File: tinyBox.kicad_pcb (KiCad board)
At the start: 2 copper layers, 29 x 20 mm, 15 parts, among them J1 USB_B_Micro, SW1 SW_DIP_x01, U1 ATSAMD21E15A-M, U2 AP2112K-3.3

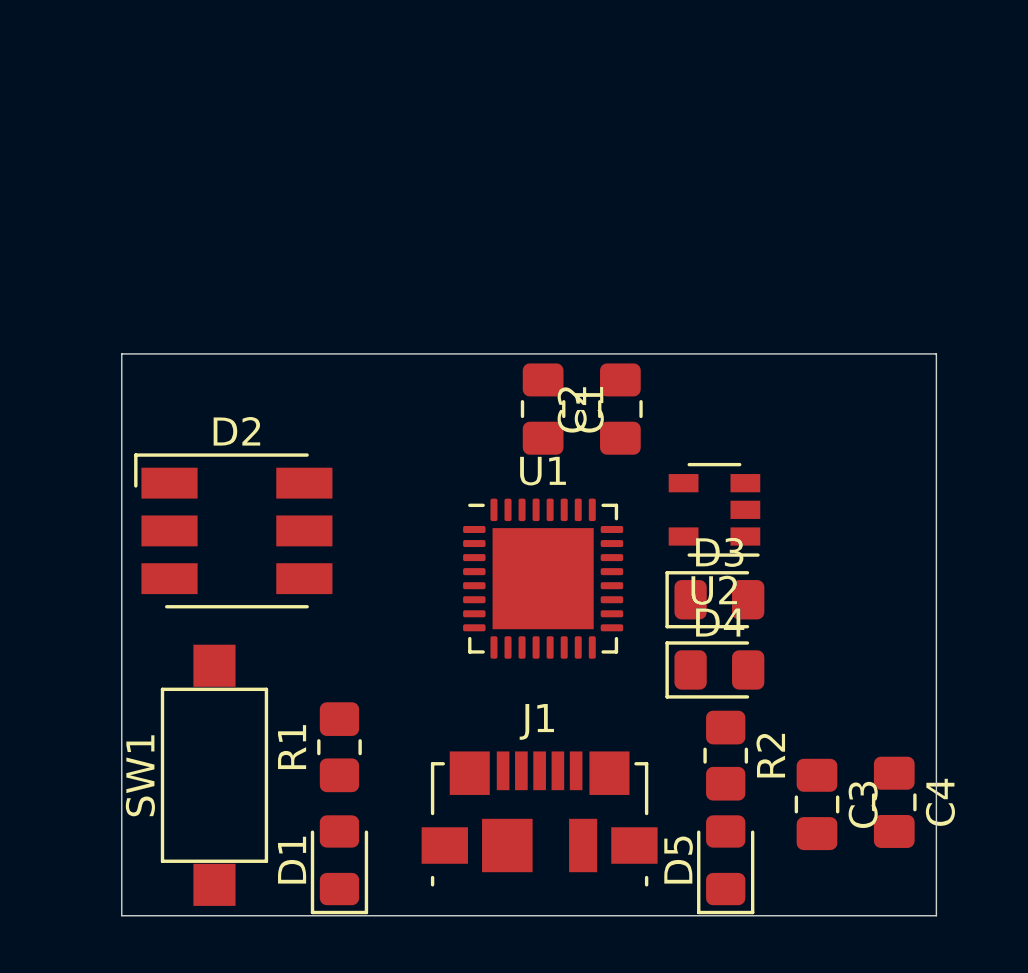
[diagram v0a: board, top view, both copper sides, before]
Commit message: Add files via upload
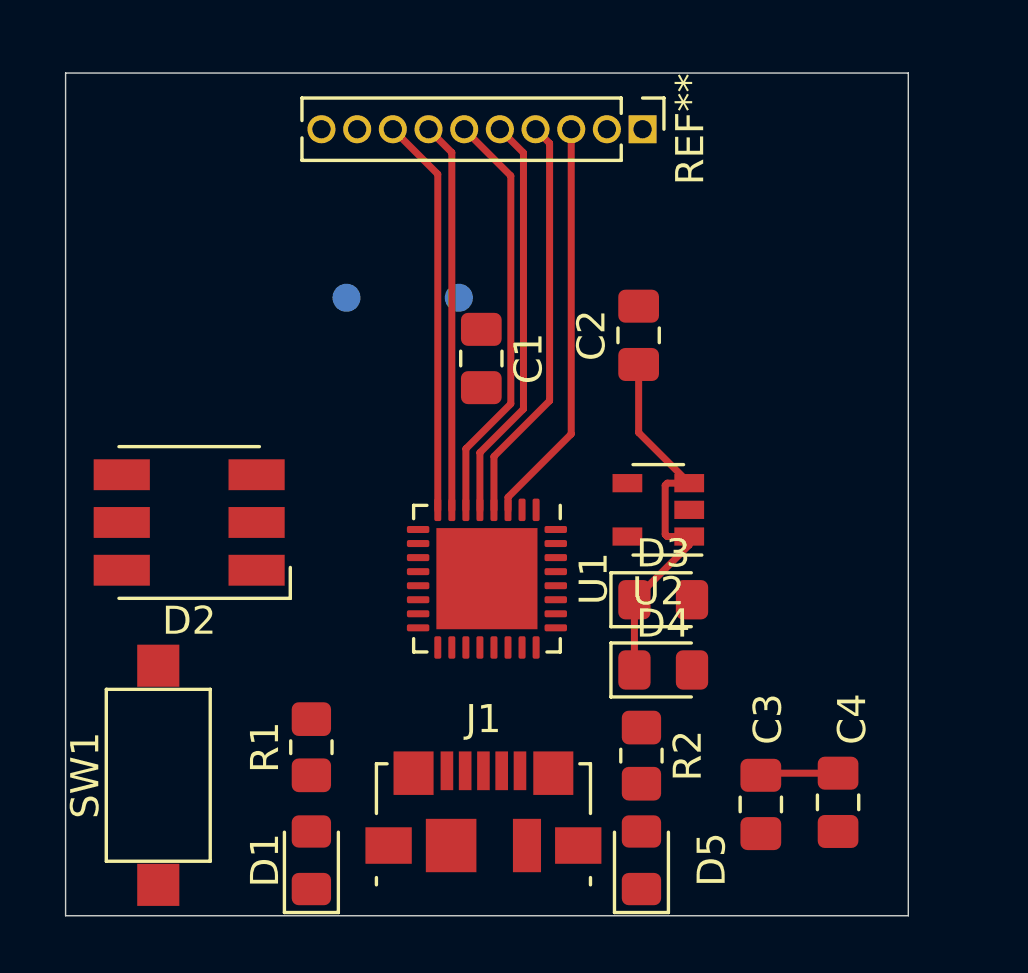
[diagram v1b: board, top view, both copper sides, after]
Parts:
- added REF**: TestPoint_Pad_D1.0mm, TestPoint:TestPoint_Pad_D1.0mm, B.Cu at (124.0, 78.0)
- added REF**: TestPoint_Pad_D1.0mm, TestPoint:TestPoint_Pad_D1.0mm, B.Cu at (120.0, 78.0)
- added REF**: PinHeader_1x10_P1.27mm_Vertical, Connector_PinHeader_1.27mm:PinHeader_1x10_P1.27mm_Vertical, F.Cu at (130.5, 72.0)
- moved D5 3.00 mm to (130.5, 98.0)
- moved R2 3.00 mm to (130.5, 94.3)
- moved C1 2.84 mm to (124.8, 80.2)
- moved C2 2.70 mm to (130.4, 79.3)
- moved C3 2.00 mm to (134.8, 96.0)
- moved C4 2.00 mm to (137.5, 96.0)
- moved D3 2.00 mm to (131.3, 88.8)
- moved D4 2.00 mm to (131.3, 91.2)
- moved J1 2.00 mm to (124.9, 96.3)
- moved SW1 2.00 mm to (113.3, 95.0)
- moved U1 2.00 mm to (125.0, 88.0), turned to 270 degrees
- moved U2 2.00 mm to (131.1, 85.5)
- moved D2 1.73 mm to (114.4, 86.0), turned to 180 degrees
- moved D1 1.00 mm to (118.8, 98.0)
- moved R1 1.00 mm to (118.8, 94.0)
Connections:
- U1 pad 1: Net-(D2-Pad6) -> Net-(D2-Pad1)
- U1 pad 11: Net-(U1-Pad11) -> D6
- U1 pad 2: Net-(D2-Pad5) -> Net-(D2-Pad2)
- U1 pad 3: Net-(U1-Pad3) -> D0_A4
- U1 pad 4: Net-(U1-Pad4) -> D1_A0
- U1 pad 5: Net-(U1-Pad5) -> D2_A1
- U1 pad 6: Net-(U1-Pad6) -> D3_A3
- U1 pad 7: Net-(U1-Pad7) -> D4_A2
- U1 pad 8: Net-(U1-Pad8) -> D5_A5
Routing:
- net D3_A3: track 0.00 -> 14.9 mm
- net D1_A0: track 0.00 -> 14.6 mm
- net D2_A1: track 0.00 -> 14.5 mm
- net D0_A4: track 0.00 -> 14.5 mm
- net D5_A5: track 0.00 -> 14.2 mm
- net Net-(C2-Pad1): track 0.00 -> 14.1 mm
- net D4_A2: track 0.00 -> 13.9 mm
- net +3V3: track 0.00 -> 2.78 mm
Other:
- board size 29 x 20 mm -> 30 x 30 mm

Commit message: Add files via upload
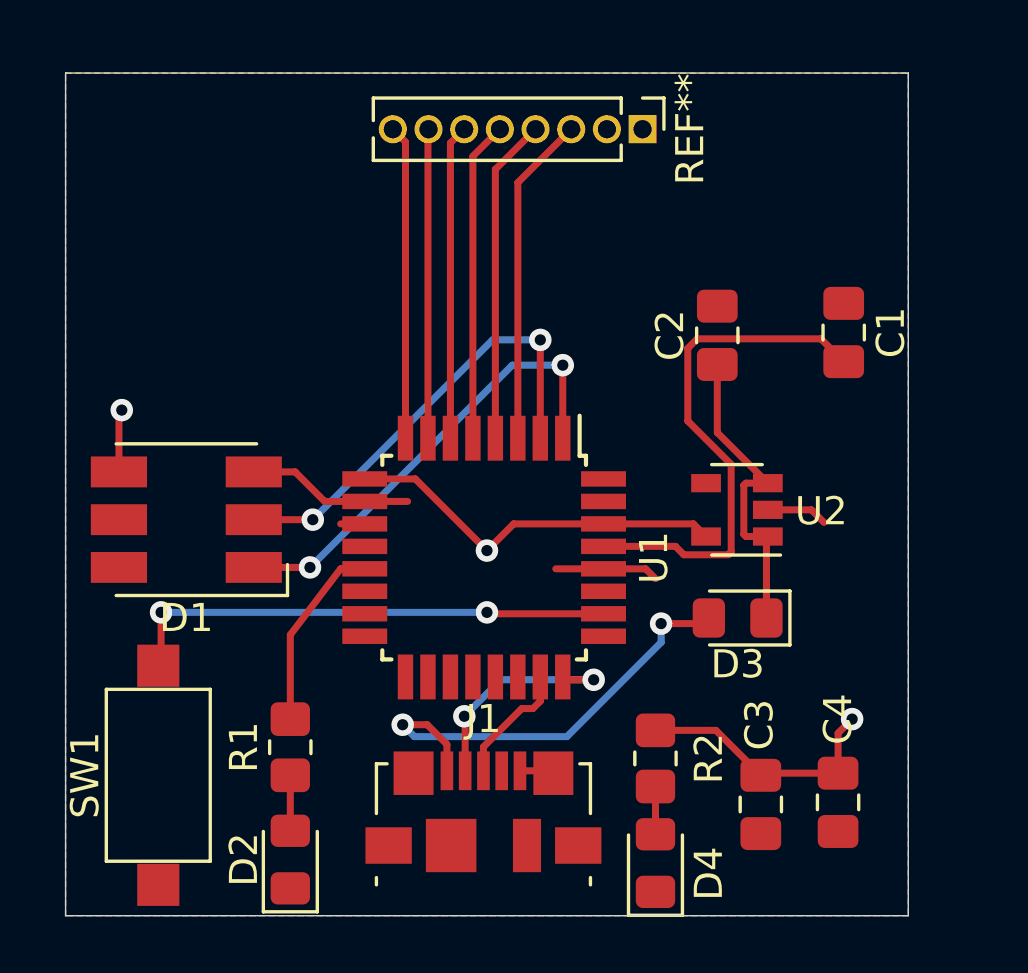
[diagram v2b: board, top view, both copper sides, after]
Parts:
- removed D5: LED, LED_SMD:LED_0805_2012Metric_Pad1.15x1.40mm_HandSolder
- removed the REF** at (124.0, 78.0)
- removed the REF** at (120.0, 78.0)
- D4: value D_Schottky -> LED; footprint Diode_SMD:D_0805_2012Metric_Pad1.15x1.40mm_HandSolder -> LED_SMD:LED_0805_2012Metric_Pad1.15x1.40mm_HandSolder
- REF**: value PinHeader_1x10_P1.27mm_Vertical -> PinHeader_1x08_P1.27mm_Vertical; footprint Connector_PinHeader_1.27mm:PinHeader_1x10_P1.27mm_Vertical -> Connector_PinHeader_1.27mm:PinHeader_1x08_P1.27mm_Vertical
- U1: value ATSAMD21E15A-M -> ATSAMD21E18A-A; footprint Package_DFN_QFN:QFN-32-1EP_5x5mm_P0.5mm_EP3.6x3.6mm -> Package_QFP:TQFP-32_7x7mm_P0.8mm
- moved C1 12.9 mm to (137.7, 79.2)
- moved D4 6.88 mm to (131.0, 98.1), turned to 90 degrees
- moved U2 2.80 mm to (133.9, 85.5)
- moved C2 2.80 mm to (133.2, 79.3)
- moved D3 2.73 mm to (133.9, 89.4), turned to 180 degrees
- moved U1 0.76 mm to (124.9, 87.2)
- moved D2 0.75 mm to (118.0, 98.0)
- moved R1 0.75 mm to (118.0, 94.0)
- moved R2 0.51 mm to (131.0, 94.4)
- moved D1 0.14 mm to (114.3, 85.9)
- renumbered D2 to D1, D1 to D2
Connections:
- D3 pad 2: VBAT -> VBUS
- D4 pad 1: Net-(C2-Pad1) -> GND
- D4 pad 2: VBUS -> Net-(D4-Pad2)
- J1 pad 1: Net-(J1-Pad1) -> VBUS
- R2 pad 2: Net-(D5-Pad2) -> Net-(D4-Pad2)
- U1 pad 11: D6 -> Net-(U1-Pad11)
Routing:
- net +3V3: track 2.78 -> 25.4 mm, vias 0 -> 3
- net Net-(C1-Pad2): track 0.00 -> 18.6 mm
- net Net-(SW1-Pad2): track 0.00 -> 17.7 mm, vias 0 -> 2
- net Net-(D1-Pad1): track 0.00 -> 16.6 mm, vias 0 -> 2
- net Net-(D1-Pad2): track 0.00 -> 16.4 mm, vias 0 -> 2
- net VBUS: track 0.00 -> 16.0 mm, vias 0 -> 2
- net GND: track 0.00 -> 13.1 mm
- net Net-(J1-Pad2): track 0.00 -> 8.24 mm, vias 0 -> 2
- net Net-(R1-Pad2): track 0.00 -> 6.81 mm
- net Net-(J1-Pad3): track 0.00 -> 4.41 mm
- net D3_A3: track 14.9 -> 11.2 mm
- net D2_A1: track 14.5 -> 11.4 mm
- net D5_A5: track 14.2 -> 11.2 mm
- net D1_A0: track 14.6 -> 11.6 mm
- net D4_A2: track 13.9 -> 11.0 mm
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- added copper zone on B.Cu, net +3V3
- added copper zone on F.Cu, net GND
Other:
- board text added: "tinyBox revised from ladyada's "trinket m0" designed in NC"

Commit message: Add files via upload
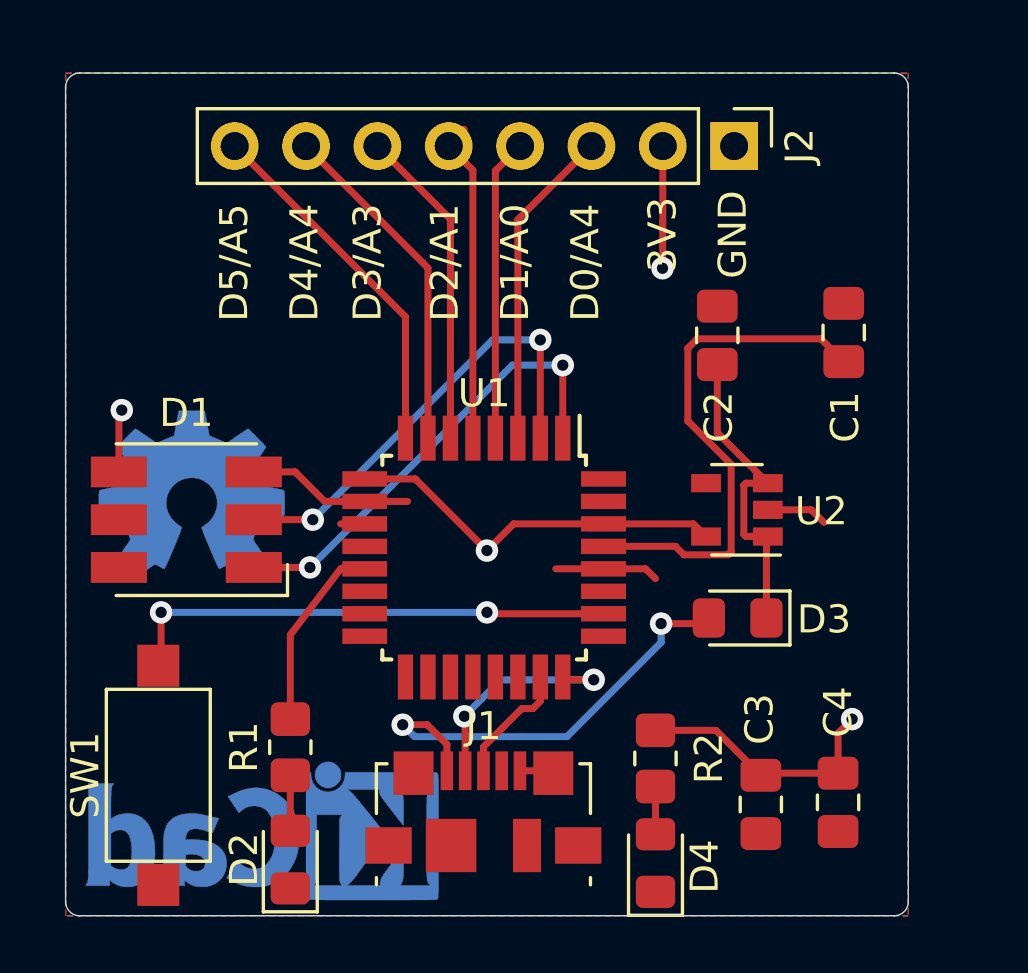
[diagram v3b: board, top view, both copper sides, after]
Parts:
- removed the REF** at (130.5, 72.0)
- added J2: Conn_01x08, Connector_PinHeader_2.54mm:PinHeader_1x08_P2.54mm_Vertical, F.Cu at (133.8, 72.6)
- added REF**: OSHW-Symbol_6.7x6mm_Copper, Symbol:OSHW-Symbol_6.7x6mm_Copper, B.Cu at (114.5, 85.0)
- added REF**: KiCad-Logo_5mm_Copper, Symbol:KiCad-Logo_5mm_Copper, B.Cu at (117.0, 97.5)
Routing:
- net 3V3: track 0.00 -> 4.35 mm, vias 0 -> 1
- net D5_A5: track 11.2 -> 12.9 mm
- net D4_A2: track 11.0 -> 12.2 mm
- net D1_A0: track 11.6 -> 10.8 mm
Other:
- outline, holes or cut-outs redrawn
- board text added: "3V3"
- board text added: "D0/A4"
- board text added: "D1/A0"
- board text added: "D2/A1"
- board text added: "D3/A3"
- board text added: "D4/A4"
- board text added: "D5/A5"
- board text added: "GND"
- board text added: "bom (all 0805 unless noted): C1, C4: 1uF C2-3: 10uF D1: APA102 D2, D4: LED D3: schottky J1: USB B micro female J2: 2.54mm, 8 prong R1: 1.5k R2: 10k U1: ATSAMD21E18A-A U2: AP2112K-3.3 SW1: DIP xxx"
